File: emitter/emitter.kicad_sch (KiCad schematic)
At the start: 16 parts, among them J1 1935174

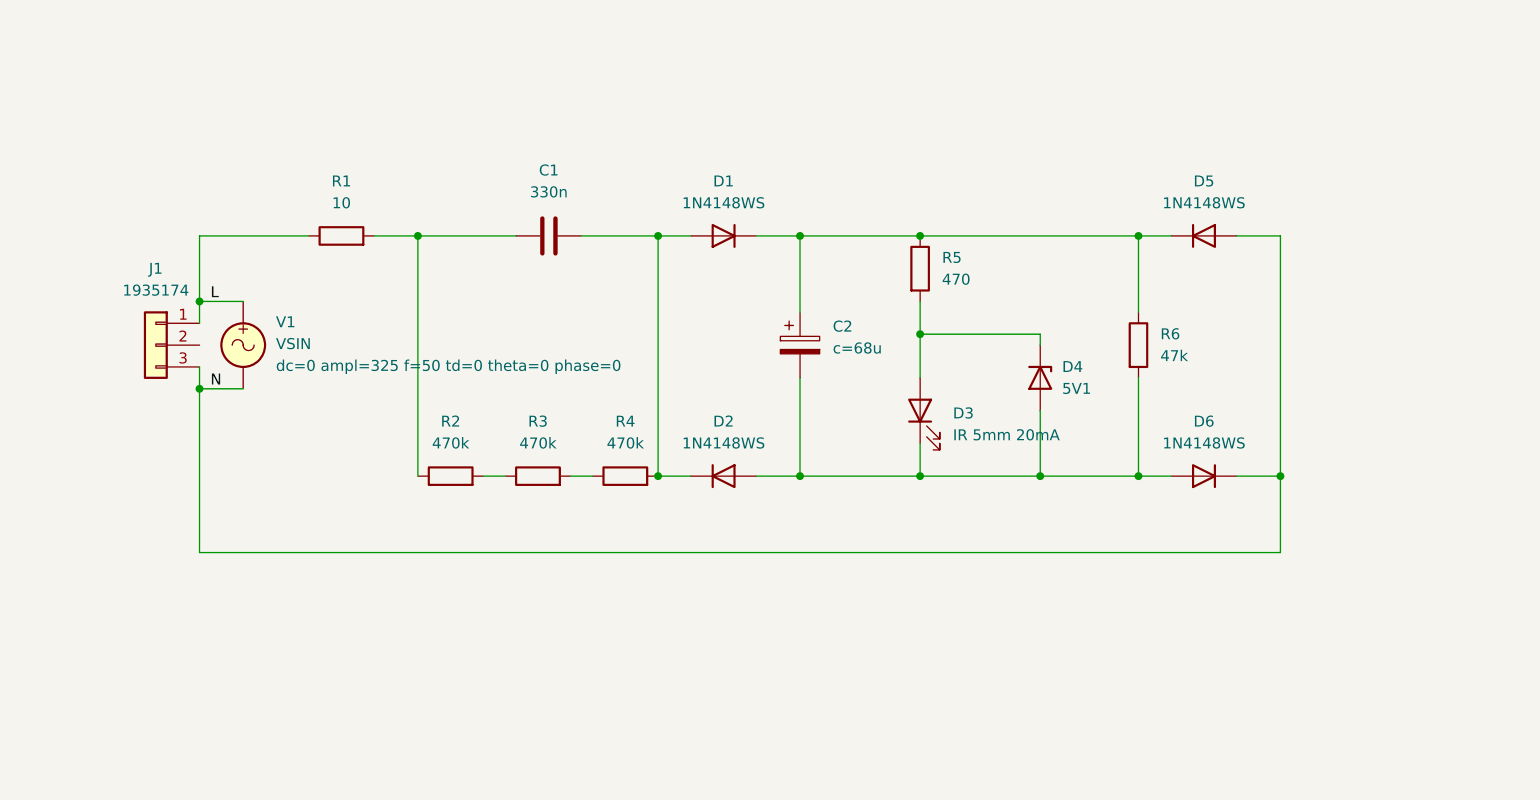
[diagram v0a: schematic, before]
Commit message: Updated rev
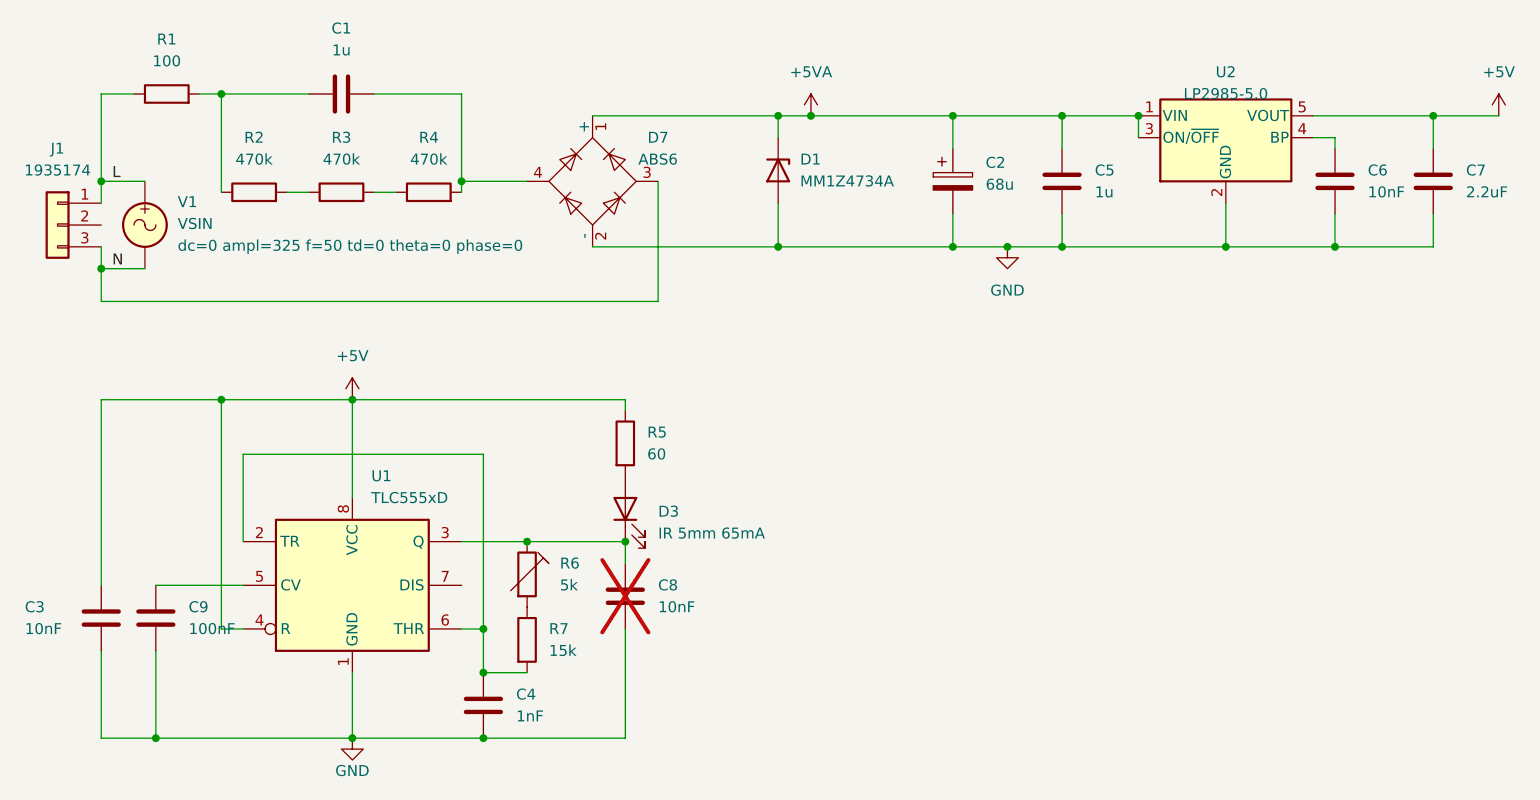
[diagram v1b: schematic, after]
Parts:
- removed D1, D2, D5, D6: 1N4148WS, Diode_SMD:D_SOD-323, symbol Diode:1N4148WS
- removed D4: 5V1, Diode_SMD:D_SOD-123F, symbol Device:D_Zener
- removed R6: 47k, Resistor_SMD:R_0805_2012Metric, symbol Device:R
- added C3, C6, C8: 10nF, Capacitor_SMD:C_0805_2012Metric, symbol Device:C
- added C4: 1nF, Capacitor_SMD:C_0805_2012Metric, symbol Device:C
- added C5: 1u, Capacitor_SMD:C_0603_1608Metric, symbol Device:C
- added C7: 2.2uF, Capacitor_SMD:C_0805_2012Metric, symbol Device:C
- added C9: 100nF, Capacitor_SMD:C_0805_2012Metric, symbol Device:C
- added D1: MM1Z4734A, Diode_SMD:D_SOD-123F, symbol Device:D_Zener
- added D7: ABS6, Diode_SMD:Diode_Bridge_Diotec_ABS, symbol Diode_Bridge:ABS6
- added R6: 5k, Potentiometer_THT:Potentiometer_Bourns_3296W_Vertical, symbol Device:R_Trim
- added R7: 15k, Resistor_SMD:R_0603_1608Metric, symbol Device:R
- added U1: TLC555xD, Package_SO:SOIC-8_3.9x4.9mm_P1.27mm, symbol Timer:TLC555xD
- added U2: LP2985-5.0, Package_TO_SOT_SMD:SOT-23-5, symbol Regulator_Linear:LP2985-5.0
- C1: value 330n -> 1u; footprint Capacitor_THT:C_Rect_L24.0mm_W7.0mm_P22.50mm_MKT -> Capacitor_THT:C_Rect_L26.5mm_W10.5mm_P22.50mm_MKS4; MPN1 WIMA:MKX2AW33304J00 -> WIMA:MKX2AW41005I00KSSD; SKU1 Conrad:1569586 - VQ -> Conrad:1569499
- C2: value ${SIM.PARAMS} -> 68u; footprint Capacitor_THT:CP_Radial_D5.0mm_P2.50mm -> Capacitor_SMD:CP_Elec_10x12.5; MPN1 Panasonic:EEU-FR1E680 -> Panasonic:50SVPF68M; SKU1 Conrad:1480946-62 -> Conrad:1675443
- D3: value IR 5mm 20mA -> IR 5mm 65mA
- J1: SKU1 Conrad:744167 - 62 -> Conrad:744167
- R1: value 10 -> 100; footprint Resistor_THT:R_Axial_DIN0516_L15.5mm_D5.0mm_P20.32mm_Horizontal -> Resistor_THT:R_Axial_DIN0516_L15.5mm_D5.0mm_P7.62mm_Vertical; MPN1 Vitrohm:CRF253-45T10R -> Vitrohm:CRF250JT-73-100RYY; SKN1 Conrad:457622 - 62 -> Conrad:2867116
- R2, R3, R4: footprint Resistor_SMD:R_0805_2012Metric -> Resistor_SMD:R_0603_1608Metric
- R5: value 470 -> 60
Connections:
- net N: now also D7.3
- net +5V: now reaches R5.1
- net +5V: now also C3.1, C7.1, U1.4 (R), U1.8 (VCC), U2.5 (VOUT); no longer C2.1
- net at D3.1 (K): now also C8.1, R6.1, U1.3 (Q); no longer C2.2
- net at C1.2, R4.2: now also D7.4
- new net: R6.2, R7.1
- new net: C9.1, U1.5 (CV)
- new net: C6.1, U2.4 (BP)
- new net: C4.1, R7.2, U1.2 (TR), U1.6 (THR)
- new net +5VA: C2.1, C5.1, D1.1 (K), D7.1 (+), U2.1 (VIN), U2.3 (ON/~{OFF})
- new net GND: C2.2, C3.2, C4.2, C5.2, C6.2, C7.2, C8.2, C9.2, D1.2 (A), D7.2 (-), U1.1 (GND), U2.2 (GND)
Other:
- moved on the sheet: C1, J1, R1, R2, R3, R4, V1
